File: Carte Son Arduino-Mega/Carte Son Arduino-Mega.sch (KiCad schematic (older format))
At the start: 18 parts, among them J1 AudioJack3, U1 CPCB_YM2413B, U2 LMC660, Y1 Crystal

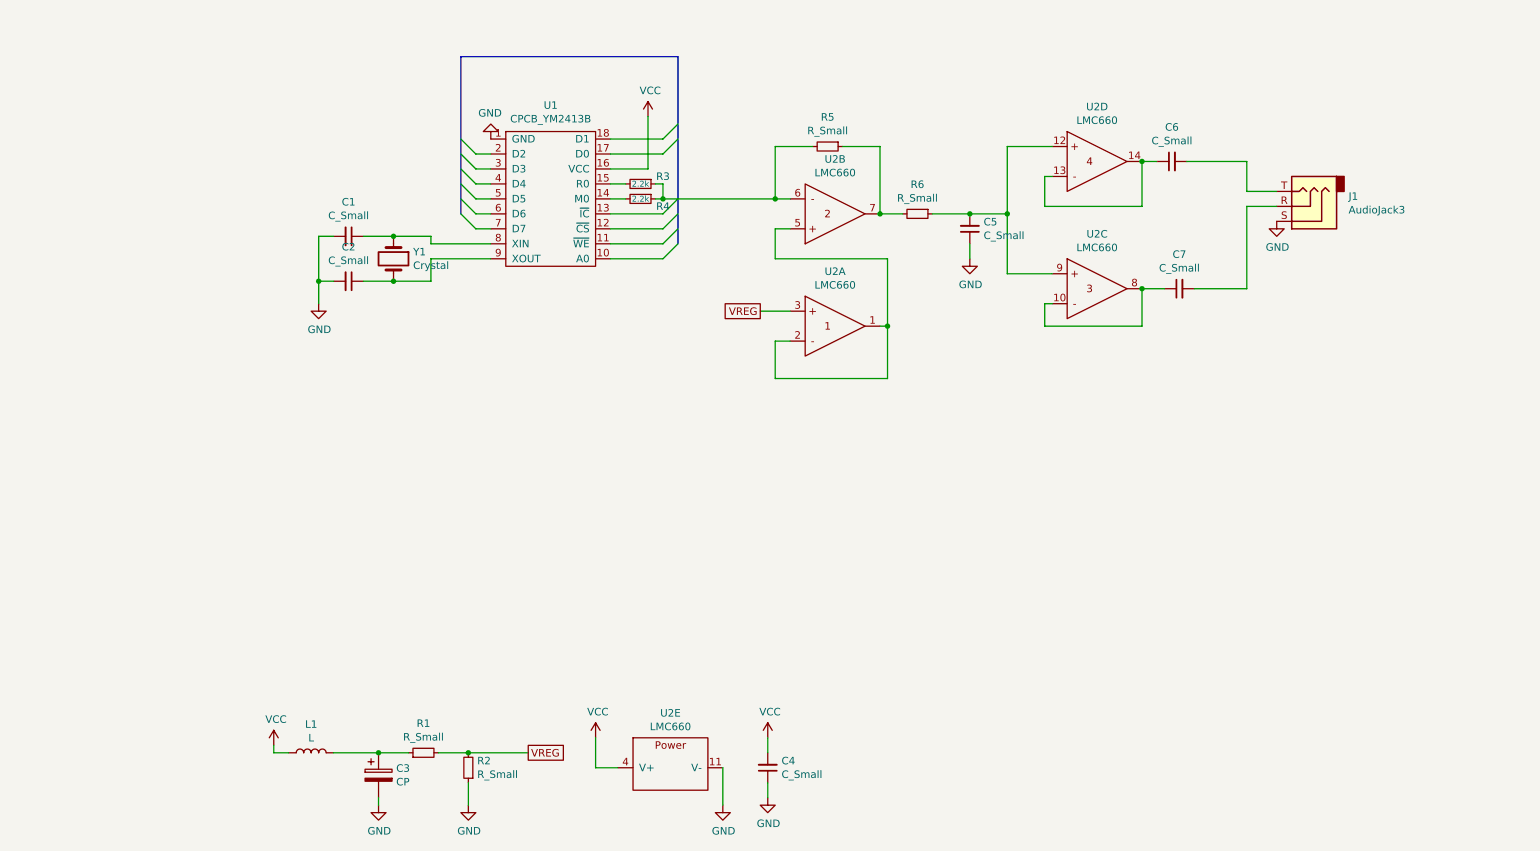
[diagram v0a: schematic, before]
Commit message: debut cours n°18
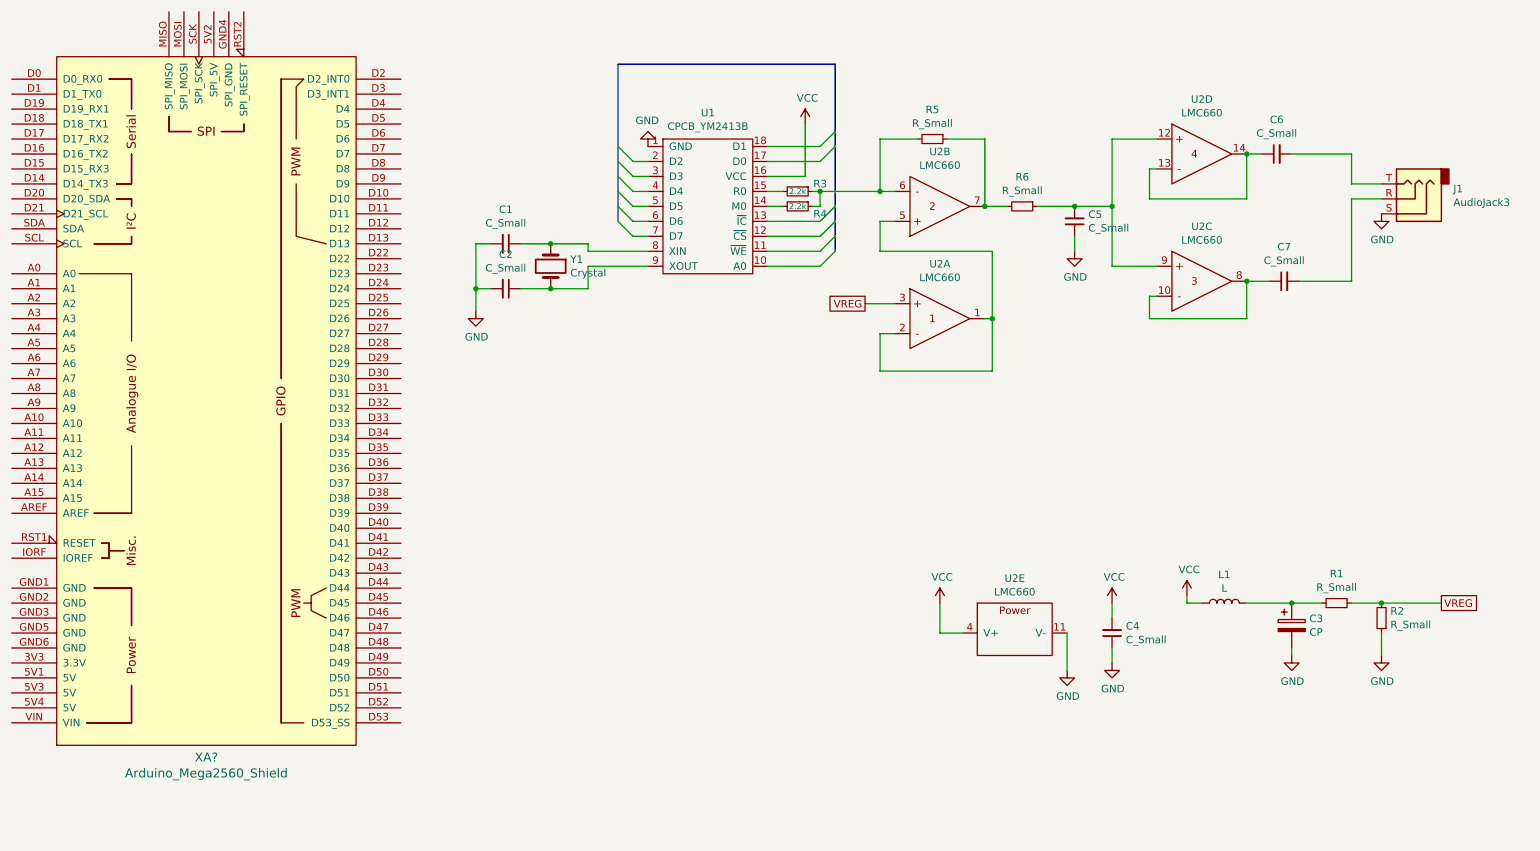
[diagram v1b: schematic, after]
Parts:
- added XA?: Arduino_Mega2560_Shield, symbol arduino:Arduino_Mega2560_Shield
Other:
- moved on the sheet: C1, C2, C3, C4, C5, C6, C7, J1, L1, R1, R2, R3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
